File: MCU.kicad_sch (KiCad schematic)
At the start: 39 parts, among them J301 SWD, J302 USB4085-GF-A_REVA4, SW301 SW_SPDT, U301 STM32F405RGT6, U302 USBLC6-2SC6, Y301 16MHz

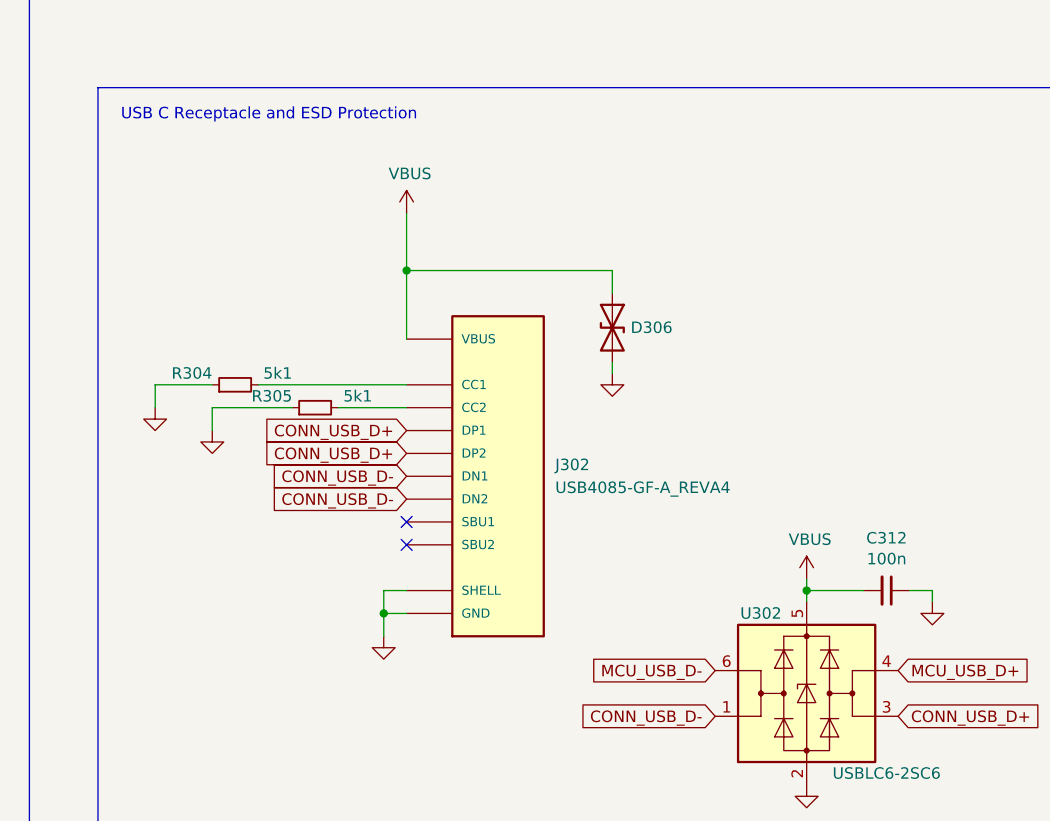
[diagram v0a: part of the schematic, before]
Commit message: sdighsidgh
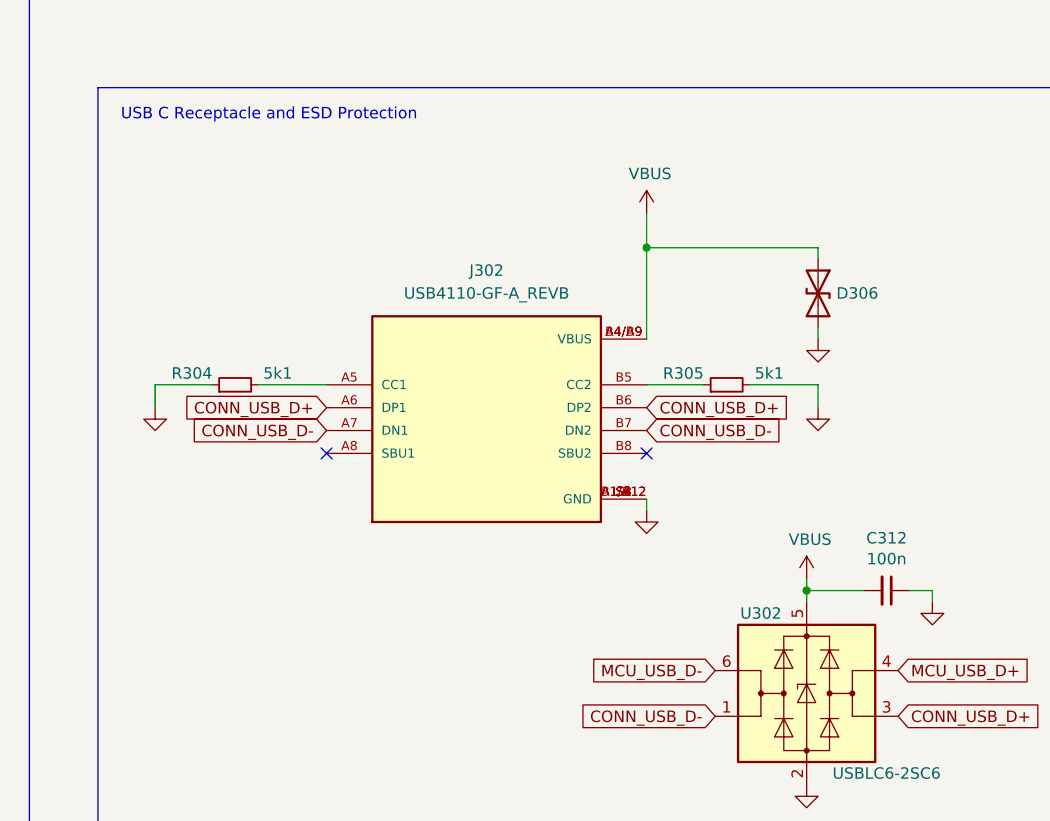
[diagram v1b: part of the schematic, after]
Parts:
- removed J302: USB4085-GF-A_REVA4, SnapEDA Library:GCT_USB4085-GF-A_REVA4, symbol USB4085-GF-A:USB4085-GF-A_REVA4
- added J302: USB4110-GF-A_REVB, SnapEDA Library:GCT_USB4110-GF-A_REVB, symbol USB4110:USB4110-GF-A_REVB
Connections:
- net CONN_USB_D+: now also J302.A6 (DP1), J302.B6 (DP2)
- net CONN_USB_D-: now also J302.A7 (DN1), J302.B7 (DN2)
- net GND: now also R305.2, J302.A1/B12 (GND), J302.B1/A12 (GND), J302.S1 (GND), J302.S2 (GND), J302.S3 (GND), J302.S4 (GND); no longer R305.1
- net VBUS: now also J302.A4/B9 (VBUS), J302.B4/A9 (VBUS)
- net at R304.2: now also J302.A5 (CC1)
- new net: J302.B5 (CC2), R305.1
